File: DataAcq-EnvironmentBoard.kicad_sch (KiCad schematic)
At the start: 25 parts, among them J1 CAN Output, J2 CAN Input, U1 SHT45, U2 FS3000-1005, U3 LMT87DCK, U4 Daughterboard Connector

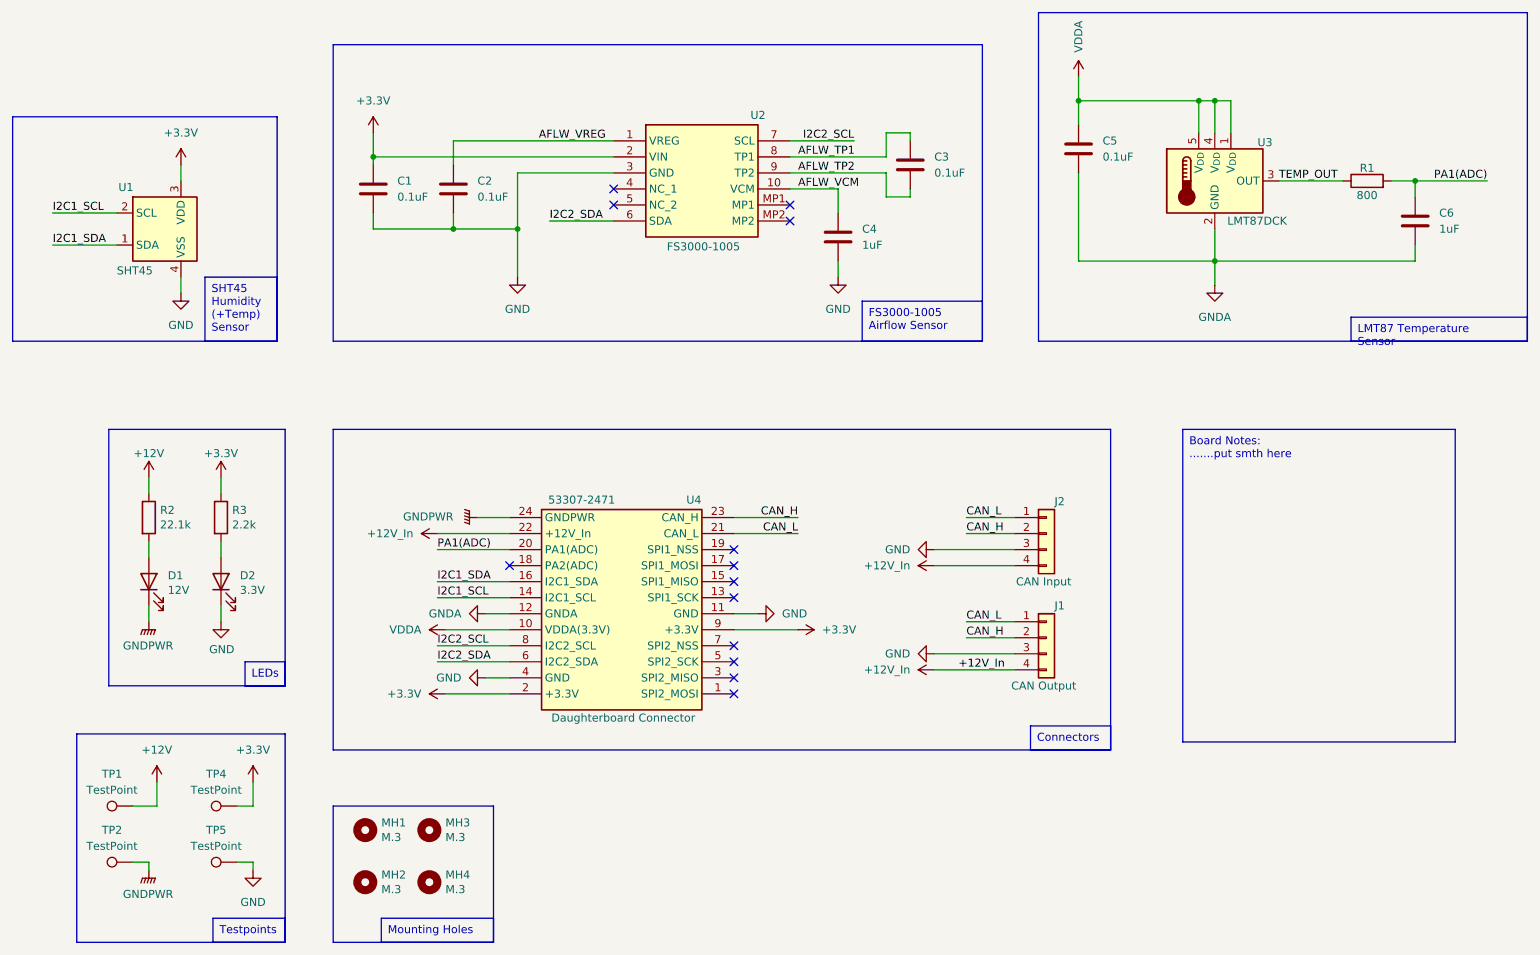
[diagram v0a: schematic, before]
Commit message: test points
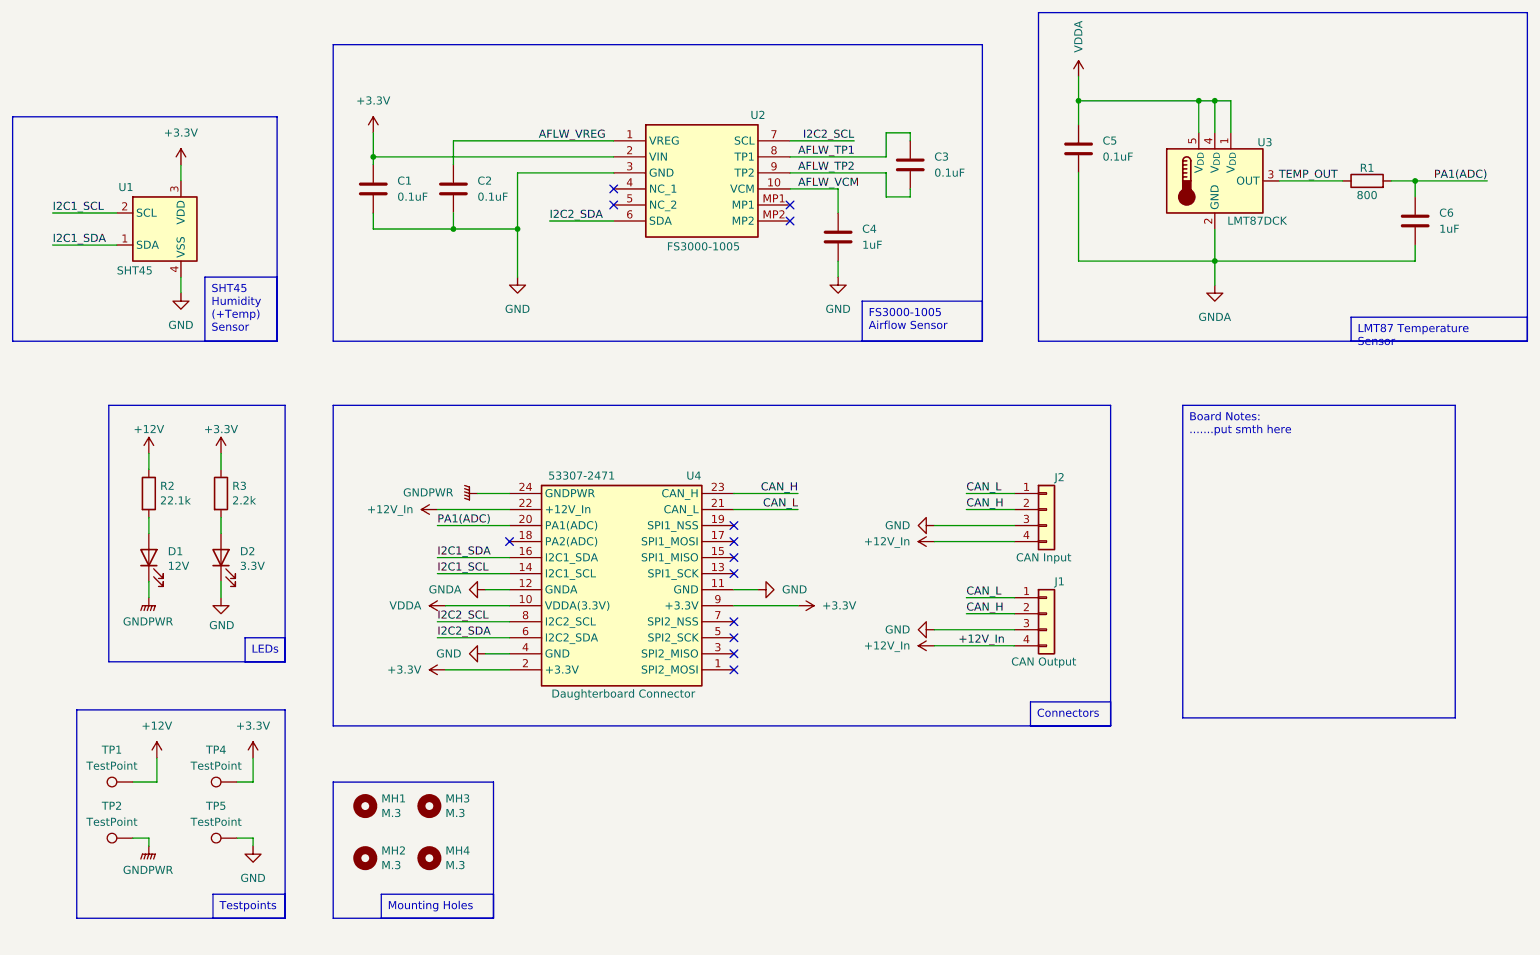
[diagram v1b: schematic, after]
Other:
- moved on the sheet: D1, D2, J1, J2, MH1, MH2, MH3, MH4, R2, R3, TP1, TP2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
